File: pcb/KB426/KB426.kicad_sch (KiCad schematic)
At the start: 129 parts, among them SW1 SW_Push_45deg, SW10 SW_Push_45deg, SW11 SW_Push_45deg, SW12 SW_Push_45deg, SW13 SW_Push_45deg, SW14 SW_Push_45deg, SW15 SW_Push_45deg, SW16 SW_Push_45deg, SW17 SW_Push_45deg, SW18 SW_Push_45deg, SW19 SW_Push_45deg, SW2 SW_Push_45deg, SW20 SW_Push_45deg, SW21 SW_Push_45deg, SW22 SW_Push_45deg, SW23 SW_Push_45deg, SW24 SW_Push_45deg, SW25 SW_Push_45deg, SW26 SW_Push_45deg, SW27 SW_Push_45deg, SW28 SW_Push_45deg, SW29 SW_Push_45deg, SW3 SW_Push_45deg, SW30 SW_Push_45deg, SW31 SW_Push_45deg, SW32 SW_Push_45deg, SW33 SW_Push_45deg, SW34 SW_Push_45deg, SW35 SW_Push_45deg, SW36 SW_Push_45deg, SW37 SW_Push_45deg, SW38 SW_Push_45deg, SW39 SW_Push_45deg, SW4 SW_Push_45deg, SW40 SW_Push_45deg, SW41 SW_Push_45deg, SW42 SW_Push_45deg, SW43 SW_Push_45deg, SW44 SW_Push_45deg, SW45 SW_Push_45deg, SW46 SW_Push_45deg, SW47 SW_Push_45deg, SW48 SW_Push_45deg, SW49 SW_Push_45deg, SW5 SW_Push_45deg, SW50 SW_Push_45deg, SW51 SW_Push_45deg, SW52 SW_Push_45deg, SW53 SW_Push_45deg, SW54 SW_Push_45deg, SW55 SW_Push_45deg, SW56 SW_Push_45deg, SW57 SW_Push_45deg, SW58 SW_Push_45deg, SW59 SW_Push_45deg, SW6 SW_Push_45deg, SW60 SW_Push_45deg, SW61 SW_Push_45deg, SW62 SW_Push_45deg, SW63 SW_Push_45deg, SW64 SW_Push_45deg, SW7 SW_Push_45deg, SW8 SW_Push_45deg, SW9 SW_Push_45deg, U1 Pico

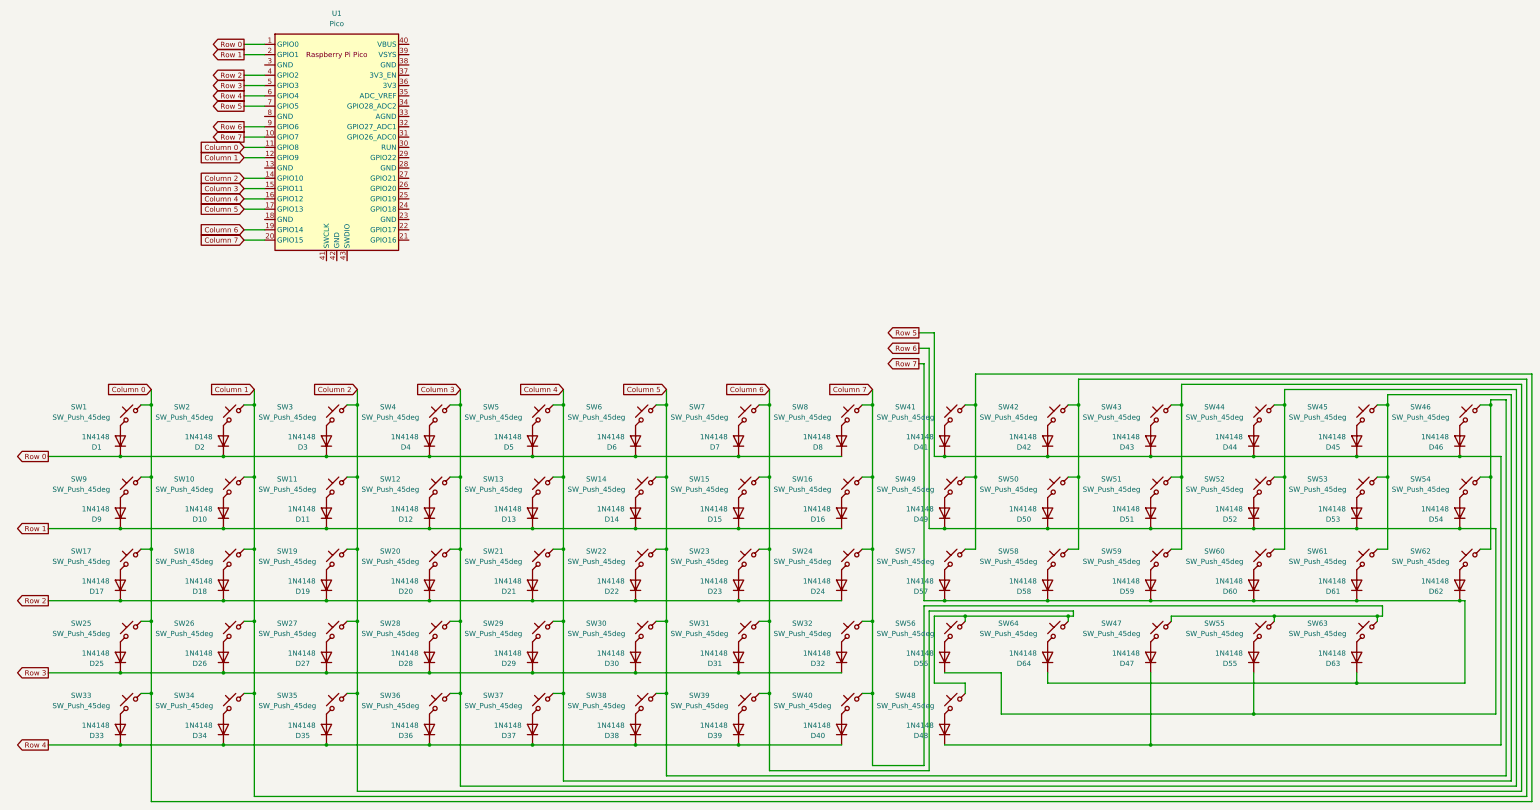
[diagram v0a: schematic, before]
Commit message: + update sch and pcb
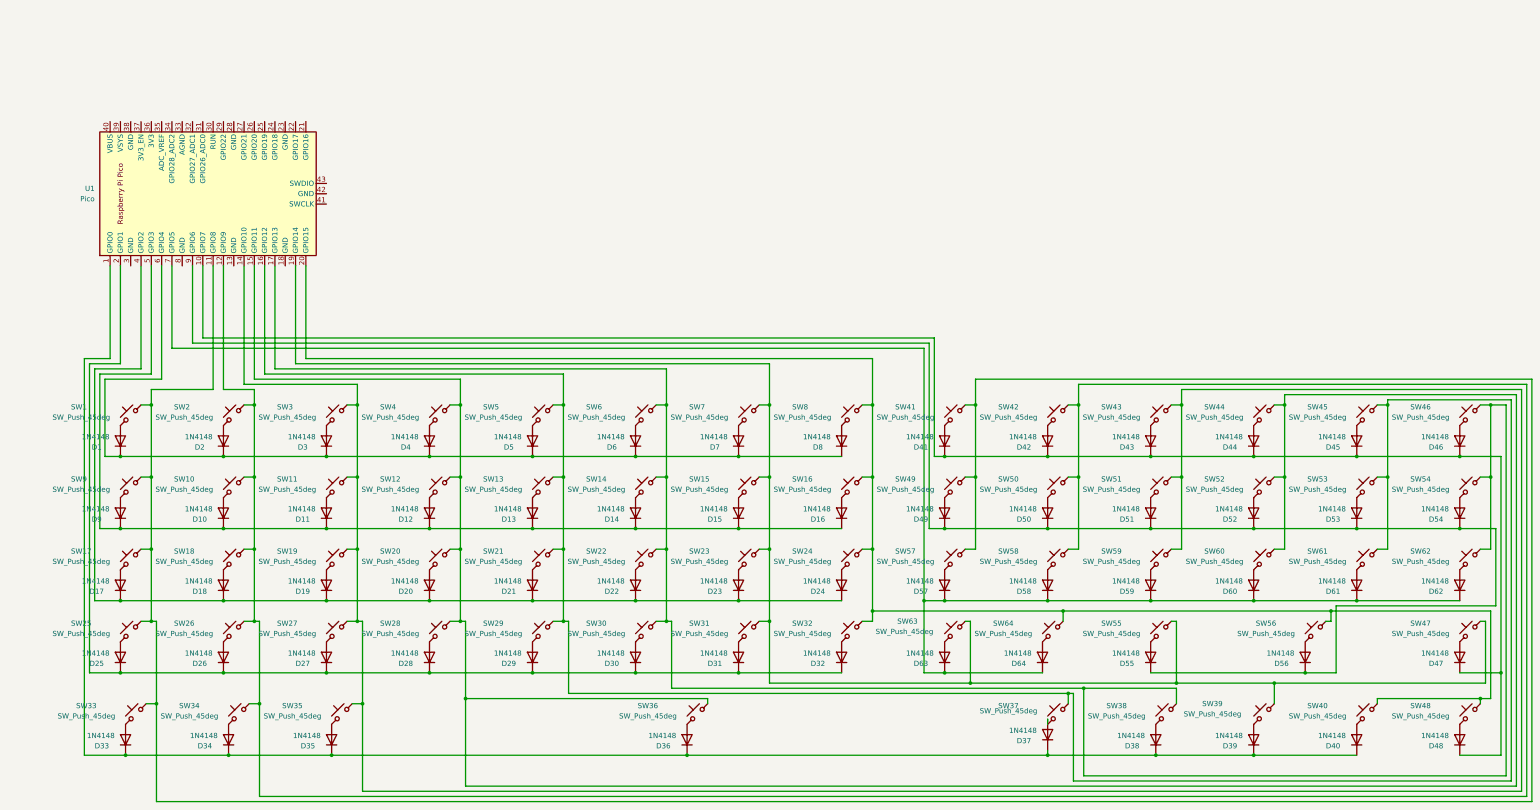
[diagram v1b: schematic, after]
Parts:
- SW47: footprint PCM_Switch_Keyboard_Cherry_MX:SW_Cherry_MX_PCB_2.00u -> PCM_Switch_Keyboard_Cherry_MX:SW_Cherry_MX_PCB_1.00u
- SW56: footprint PCM_Switch_Keyboard_Cherry_MX:SW_Cherry_MX_PCB_1.00u -> PCM_Switch_Keyboard_Cherry_MX:SW_Cherry_MX_PCB_2.00u
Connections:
- net Column 0: no longer names the net of SW1.2, SW17.2, SW25.2, SW33.2, SW41.2, SW49.2, SW57.2, SW9.2, U1.11 (GPIO8)
- net Column 1: no longer names the net of SW10.2, SW18.2, SW2.2, SW26.2, SW34.2, SW42.2, SW50.2, SW58.2, U1.12 (GPIO9)
- net Column 2: no longer names the net of SW11.2, SW19.2, SW27.2, SW3.2, SW35.2, SW43.2, SW51.2, SW59.2, U1.14 (GPIO10)
- net Column 3: no longer names the net of SW12.2, SW20.2, SW28.2, SW36.2, SW4.2, SW44.2, SW52.2, SW60.2, U1.15 (GPIO11)
- net Column 4: no longer names the net of SW13.2, SW21.2, SW29.2, SW37.2, SW45.2, SW5.2, SW53.2, SW61.2, U1.16 (GPIO12)
- net Column 5: no longer names the net of SW14.2, SW22.2, SW30.2, SW38.2, SW46.2, SW54.2, SW6.2, SW62.2, U1.17 (GPIO13)
- net Column 6: no longer names the net of SW15.2, SW23.2, SW31.2, SW39.2, SW7.2, U1.19 (GPIO14)
- net Column 6: now also SW47.2, SW55.2, SW63.2; no longer SW48.2, SW56.2, SW64.2
- net Column 7: no longer names the net of SW16.2, SW24.2, SW32.2, SW40.2, SW8.2, U1.20 (GPIO15)
- net Column 7: now also SW48.2, SW56.2, SW64.2; no longer SW47.2, SW55.2, SW63.2
- net Row 0: no longer names the net of D1.1 (K), D2.1 (K), D3.1 (K), D4.1 (K), D5.1 (K), D6.1 (K), D7.1 (K), D8.1 (K)
- net Row 0: now also U1.6 (GPIO4); no longer U1.1 (GPIO0)
- net Row 1: no longer names the net of D10.1 (K), D11.1 (K), D12.1 (K), D13.1 (K), D14.1 (K), D15.1 (K), D16.1 (K), D9.1 (K)
- net Row 1: now also U1.5 (GPIO3); no longer U1.2 (GPIO1)
- net Row 2: no longer names the net of D17.1 (K), D18.1 (K), D19.1 (K), D20.1 (K), D21.1 (K), D22.1 (K), D23.1 (K), D24.1 (K), U1.4 (GPIO2)
- net Row 3: no longer names the net of D25.1 (K), D26.1 (K), D27.1 (K), D28.1 (K), D29.1 (K), D30.1 (K), D31.1 (K), D32.1 (K)
- net Row 3: now also U1.2 (GPIO1); no longer U1.5 (GPIO3)
- net Row 4: no longer names the net of D33.1 (K), D34.1 (K), D35.1 (K), D36.1 (K), D37.1 (K), D38.1 (K), D39.1 (K), D40.1 (K)
- net Row 4: now also U1.1 (GPIO0); no longer U1.6 (GPIO4)
- net Row 5: no longer names the net of D41.1 (K), D42.1 (K), D43.1 (K), D44.1 (K), D45.1 (K), D46.1 (K), D47.1 (K), D48.1 (K)
- net Row 5: now also U1.10 (GPIO7); no longer U1.7 (GPIO5)
- net Row 6: no longer names the net of D49.1 (K), D50.1 (K), D51.1 (K), D52.1 (K), D53.1 (K), D54.1 (K), D55.1 (K), D56.1 (K), U1.9 (GPIO6)
- net Row 7: no longer names the net of D57.1 (K), D58.1 (K), D59.1 (K), D60.1 (K), D61.1 (K), D62.1 (K), D63.1 (K), D64.1 (K)
- net Row 7: now also U1.7 (GPIO5); no longer U1.10 (GPIO7)
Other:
- moved on the sheet: D33, D34, D35, D36, D37, D38, D39, D40, D47, D48, D55, D56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
